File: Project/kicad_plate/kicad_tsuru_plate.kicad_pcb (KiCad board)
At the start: 2 copper layers, 209.6 x 57.2 mm, 4 parts

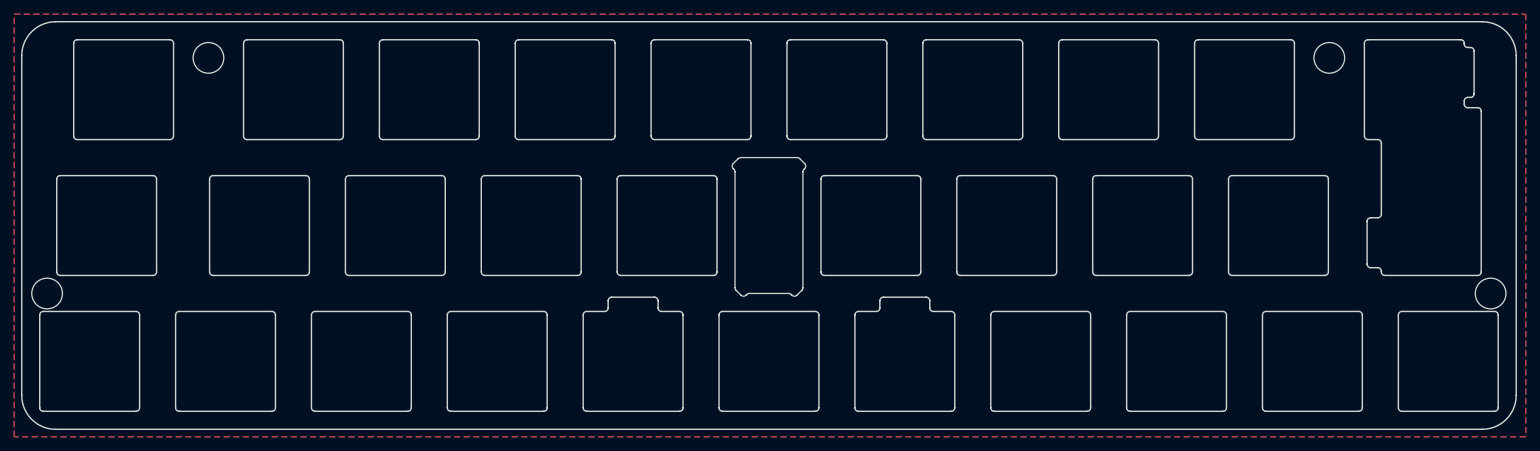
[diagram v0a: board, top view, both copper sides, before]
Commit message: plate update
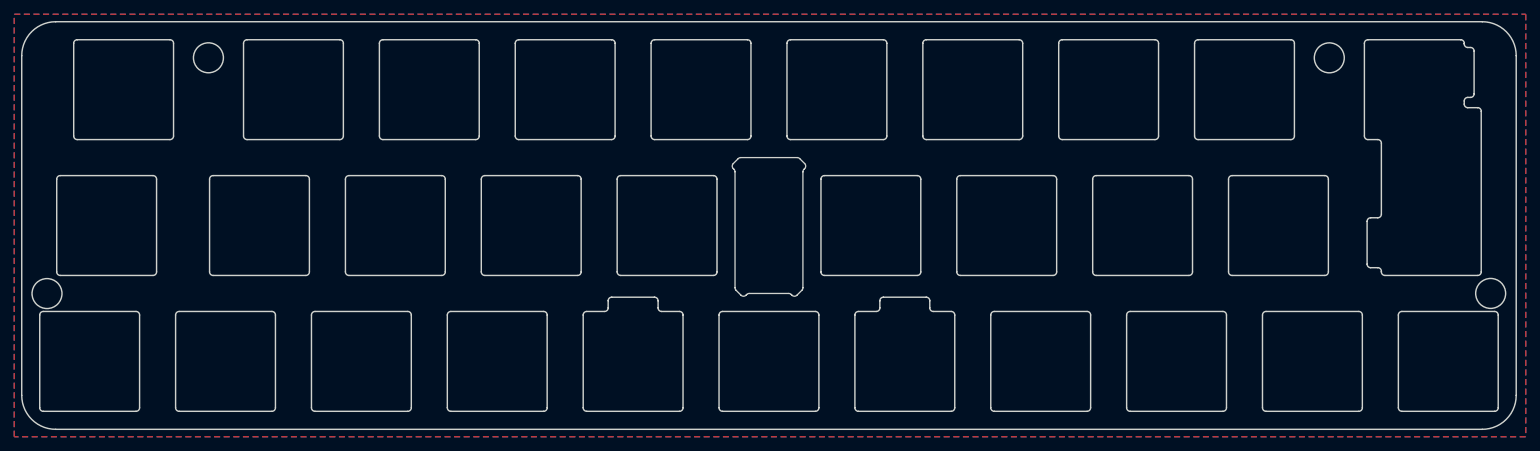
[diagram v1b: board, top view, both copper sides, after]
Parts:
- removed REF** (x4): MountingHole_4.3mm_M4, MountingHole:MountingHole_4.3mm_M4
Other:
- outline, holes or cut-outs redrawn
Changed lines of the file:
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@@
   )
   (net 0 "")
-  (footprint "MountingHole:MountingHole_4.3mm_M4" (layer "F.Cu")
-    (at 215.837837 58.601934)
-    (descr "Mounting Hole 4.3mm, no annular, M4")
-    (tags "mounting hole 4.3mm no annular m4")
-    (attr exclude_from_pos_files exclude_from_bom)
-    (fp_text reference "REF**" (at 0 -5.3) (layer "F.SilkS") hide
-        (effects (font (size 1 1) (thickness 0.15)))
-    )
-    (fp_text value "MountingHole_4.3mm_M4" (at 0 5.3) (layer "F.Fab")
-        (effects (font (size 1 1) (thickness 0.15)))
-    )
-    (fp_text user "${REFERENCE}" (at 0 0) (layer "F.Fab")
-        (effects (font (size 1 1) (thickness 0.15)))
-    )
-    (fp_circle (center 0 0) (end 4.3 0)
-      (stroke (width 0.15) (type solid)) (fill none) (layer "Cmts.User"))
-    (fp_circle (center 0 0) (end 4.55 0)
-      (stroke (width 0.05) (type solid)) (fill none) (layer "F.CrtYd"))
-    (pad "" np_thru_hole circle (at 0 0) (size 4.3 4.3) (drill 4.3) (layers "*.Cu" "*.Mask"))
-  )
-  (footprint "MountingHole:MountingHole_4.3mm_M4" (layer "F.Cu")
-    (at 36.053009 91.641861)
-    (descr "Mounting Hole 4.3mm, no annular, M4")
-    (tags "mounting hole 4.3mm no annular m4")
-    (attr exclude_from_pos_files exclude_from_bom)
-    (fp_text reference "REF**" (at 0 -5.3) (layer "B.SilkS") hide
-        (effects (font (size 1 1) (thickness 0.15)) (justify mirror))
-    )
-    (fp_text value "MountingHole_4.3mm_M4" (at 0 5.3) (layer "F.Fab")
-        (effects (font (size 1 1) (thickness 0.15)))
-    )
-    (fp_text user "${REFERENCE}" (at 0 0) (layer "F.Fab")
-        (effects (font (size 1 1) (thickness 0.15)))
-    )
-    (fp_circle (center 0 0) (end 4.3 0)
-      (stroke (width 0.15) (type solid)) (fill none) (layer "Cmts.User"))
-    (fp_circle (center 0 0) (end 4.55 0)
-      (stroke (width 0.05) (type solid)) (fill none) (layer "F.CrtYd"))
-    (pad "" np_thru_hole circle (at 0 0) (size 4.3 4.3) (drill 4.3) (layers "*.Cu" "*.Mask"))
-  )
-  (footprint "MountingHole:MountingHole_4.3mm_M4" (layer "F.Cu")
-    (at 58.674941 58.601934)
-    (descr "Mounting Hole 4.3mm, no annular, M4")
-    (tags "mounting hole 4.3mm no annular m4")
-    (attr exclude_from_pos_files exclude_from_bom)
-    (fp_text reference "REF**" (at 0 -5.3) (layer "F.SilkS") hide
-        (effects (font (size 1 1) (thickness 0.15)))
-    )
-    (fp_text value "MountingHole_4.3mm_M4" (at 0 5.3) (layer "F.Fab")
-        (effects (font (size 1 1) (thickness 0.15)))
-    )
-    (fp_text user "${REFERENCE}" (at 0 0) (layer "F.Fab")
-        (effects (font (size 1 1) (thickness 0.15)))
-    )
-    (fp_circle (center 0 0) (end 4.3 0)
-      (stroke (width 0.15) (type solid)) (fill none) (layer "Cmts.User"))
-    (fp_circle (center 0 0) (end 4.55 0)
-      (stroke (width 0.05) (type solid)) (fill none) (layer "F.CrtYd"))
-    (pad "" np_thru_hole circle (at 0 0) (size 4.3 4.3) (drill 4.3) (layers "*.Cu" "*.Mask"))
-  )
-  (footprint "MountingHole:MountingHole_4.3mm_M4" (layer "F.Cu")
-    (at 238.459769 91.641861)
-    (descr "Mounting Hole 4.3mm, no annular, M4")
-    (tags "mounting hole 4.3mm no annular m4")
-    (attr exclude_from_pos_files exclude_from_bom)
-    (fp_text reference "REF**" (at 0 -5.3) (layer "F.SilkS") hide
-        (effects (font (size 1 1) (thickness 0.15)))
-    )
-    (fp_text value "MountingHole_4.3mm_M4" (at 0 5.3) (layer "F.Fab")
-        (effects (font (size 1 1) (thickness 0.15)))
-    )
-    (fp_text user "${REFERENCE}" (at 0 0) (layer "F.Fab")
-        (effects (font (size 1 1) (thickness 0.15)))
-    )
-    (fp_circle (center 0 0) (end 4.3 0)
-      (stroke (width 0.15) (type solid)) (fill none) (layer "Cmts.User"))
-    (fp_circle (center 0 0) (end 4.55 0)
-      (stroke (width 0.05) (type solid)) (fill none) (layer "F.CrtYd"))
-    (pad "" np_thru_hole circle (at 0 0) (size 4.3 4.3) (drill 4.3) (layers "*.Cu" "*.Mask"))
-  )
   (gr_arc (start 64.095434 70.058755) (mid 63.741851 69.91233) (end 63.595434 69.558755)
     (stroke (width 0.2) (type solid)) (layer "Edge.Cuts"))
@@
   (gr_arc (start 242.045434 105.921255) (mid 240.650507 109.288801) (end 237.282934 110.683755)
     (stroke (width 0.2) (type default)) (layer "Edge.Cuts"))
+  (gr_circle (center 238.461807 91.631243) (end 240.561807 91.631243)
+    (stroke (width 0.2) (type default)) (fill none) (layer "Edge.Cuts"))
   (gr_line (start 121.245434 56.058755) (end 134.245434 56.058755)
     (stroke (width 0.2) (type solid)) (layer "Edge.Cuts"))
@@
   (gr_line (start 77.595434 56.558755) (end 77.595434 69.558755)
     (stroke (width 0.2) (type solid)) (layer "Edge.Cuts"))
+  (gr_circle (center 58.673548 58.591164) (end 60.773548 58.591164)
+    (stroke (width 0.2) (type default)) (fill none) (layer "Edge.Cuts"))
   (gr_line (start 63.595434 56.558755) (end 63.595434 69.558755)
     (stroke (width 0.2) (type solid)) (layer "Edge.Cuts"))
@@
   (gr_arc (start 132.957061 72.729852) (mid 133.119269 72.621458) (end 133.310614 72.583406)
     (stroke (width 0.1) (type default)) (layer "Edge.Cuts"))
+  (gr_circle (center 36.039856 91.649977) (end 38.139856 91.649977)
+    (stroke (width 0.2) (type default)) (fill none) (layer "Edge.Cuts"))
   (gr_arc (start 132.266434 74.127585) (mid 132.119926 73.77402) (end 132.266435 73.420478)
     (stroke (width 0.1) (type default)) (layer "Edge.Cuts"))
@@
   (gr_arc (start 187.920434 108.158755) (mid 187.566851 108.01233) (end 187.420434 107.658755)
     (stroke (width 0.2) (type solid)) (layer "Edge.Cuts"))
+  (gr_circle (center 215.836048 58.596763) (end 217.936048 58.596763)
+    (stroke (width 0.2) (type default)) (fill none) (layer "Edge.Cuts"))
   (gr_line (start 220.757934 56.558755) (end 220.757934 69.558755)
     (stroke (width 0.2) (type solid)) (layer "Edge.Cuts"))
